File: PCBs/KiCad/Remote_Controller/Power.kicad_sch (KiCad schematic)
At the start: 25 parts

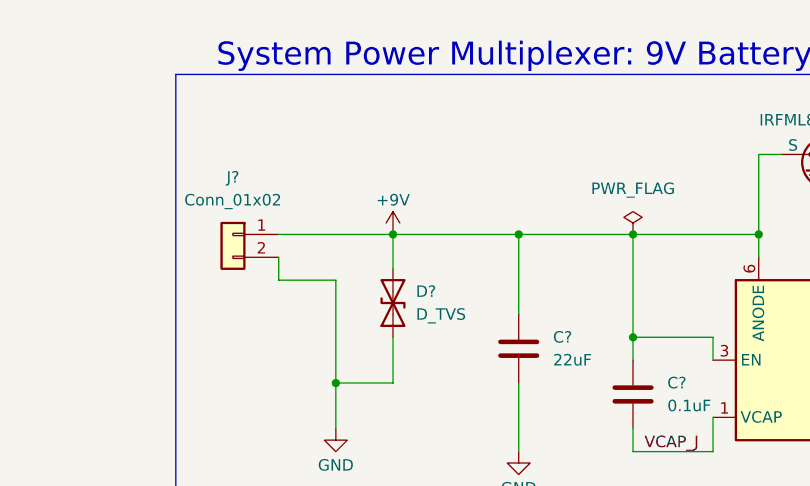
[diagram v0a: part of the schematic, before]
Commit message: Add power switch
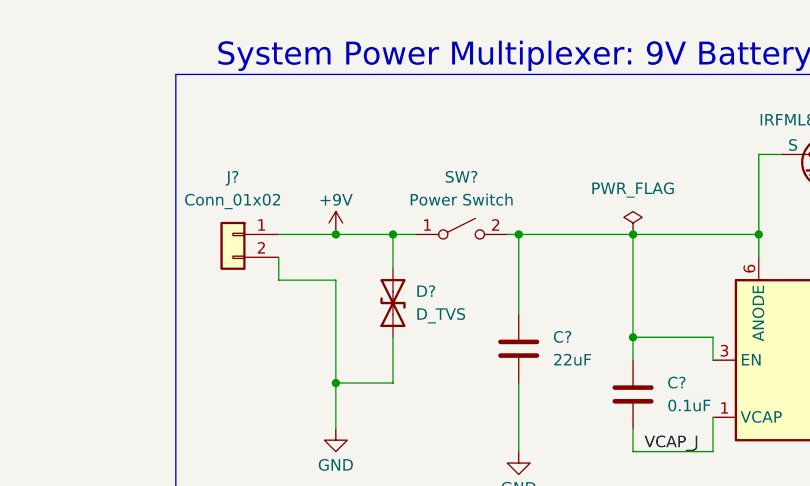
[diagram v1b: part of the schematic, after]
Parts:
- added SW?: Power Switch, symbol Switch:SW_SPST
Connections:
- net +9V: now also SW?.1 (A); no longer C?.1, C?.1, Q?.2 (S), U?.3 (EN), U?.6 (ANODE)
- new net: C?.1, C?.1, Q?.2 (S), SW?.2 (B), U?.3 (EN), U?.6 (ANODE)
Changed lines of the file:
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@@
 	(paper "A4")
 	(junction
-		(at 130.81 170.18)
+		(at 116.84 40.64)
 		(diameter 0)
 		(color 0 0 0 0)
 	)
 	(junction
-		(at 26.67 148.59)
+		(at 130.81 170.18)
 		(diameter 0)
 		(color 0 0 0 0)
 	)
 	(junction
-		(at 143.51 40.64)
+		(at 26.67 148.59)
 		(diameter 0)
 		(color 0 0 0 0)
 	)
 	(junction
-		(at 238.76 55.88)
+		(at 143.51 40.64)
 		(diameter 0)
 		(color 0 0 0 0)
 	)
 	(junction
-		(at 116.84 40.64)
+		(at 238.76 55.88)
 		(diameter 0)
 		(color 0 0 0 0)
@@
 	)
 	(junction
-		(at 102.87 40.64)
-		(diameter 0)
-		(color 0 0 0 0)
-	)
-	(junction
 		(at 106.68 148.59)
 		(diameter 0)
@@
 	)
 	(junction
+		(at 96.52 40.64)
+		(diameter 0)
+		(color 0 0 0 0)
+	)
+	(junction
 		(at 116.84 148.59)
 		(diameter 0)
@@
 	)
 	(junction
+		(at 102.87 40.64)
+		(diameter 0)
+		(color 0 0 0 0)
+	)
+	(junction
 		(at 116.84 95.25)
 		(diameter 0)
@@
 	(wire
 		(pts
-			(xy 102.87 40.64) (xy 116.84 40.64)
-		)
-		(stroke
-			(width 0)
-			(type default)
-		)
-	)
-	(wire
-		(pts
 			(xy 41.91 148.59) (xy 53.34 148.59)
 		)
@@
 	(wire
 		(pts
+			(xy 115.57 40.64) (xy 116.84 40.64)
+		)
+		(stroke
+			(width 0)
+			(type default)
+		)
+	)
+	(wire
+		(pts
 			(xy 231.14 45.72) (xy 220.98 45.72)
 		)
@@
 	(wire
 		(pts
-			(xy 90.17 40.64) (xy 102.87 40.64)
+			(xy 90.17 40.64) (xy 96.52 40.64)
 		)
 		(stroke
@@
 	(wire
 		(pts
+			(xy 102.87 40.64) (xy 105.41 40.64)
+		)
+		(stroke
+			(width 0)
+			(type default)
+		)
+	)
+	(wire
+		(pts
 			(xy 102.87 52.07) (xy 102.87 57.15)
 		)
@@
 	(wire
 		(pts
+			(xy 96.52 40.64) (xy 102.87 40.64)
+		)
+		(stroke
+			(width 0)
+			(type default)
+		)
+	)
+	(wire
+		(pts
 			(xy 220.98 55.88) (xy 238.76 55.88)
 		)
@@
 	(symbol
 		(lib_id "power:+9V")
-		(at 102.87 40.64 0)
+		(at 96.52 40.64 0)
 		(unit 1)
 		(exclude_from_sim no)
@@
 		(dnp no)
 		(property "Reference" "#PWR09"
-			(at 102.87 44.45 0)
+			(at 96.52 44.45 0)
 			(effects
 				(font
@@
 		)
 		(property "Value" "+9V"
-			(at 102.87 36.83 0)
+			(at 96.52 36.83 0)
 			(effects
 				(font
@@
 		)
 		(property "Footprint" ""
-			(at 102.87 40.64 0)
+			(at 96.52 40.64 0)
 			(effects
 				(font
@@
 		)
 		(property "Datasheet" ""
-			(at 102.87 40.64 0)
+			(at 96.52 40.64 0)
 			(effects
 				(font
@@
 		)
 		(property "Description" "Power symbol creates a global label with name \"+9V\""
-			(at 102.87 40.64 0)
+			(at 96.52 40.64 0)
 			(effects
 				(font
@@
 					(unit 1)
 				)
+			)
+		)
+	)
+	(symbol
+		(lib_id "Switch:SW_SPST")
+		(at 110.49 40.64 0)
+		(unit 1)
+		(exclude_from_sim no)
+		(in_bom yes)
+		(on_board yes)
+		(dnp no)
+		(fields_autoplaced yes)
+		(property "Reference" "SW?"
+			(at 110.49 34.29 0)
+			(effects
+				(font
+					(size 1.27 1.27)
+				)
+			)
+		)
+		(property "Value" "Power Switch"
+			(at 110.49 36.83 0)
+			(effects
+				(font
+					(size 1.27 1.27)
+				)
+			)
+		)
+		(property "Footprint" ""
+			(at 110.49 40.64 0)
+			(effects
+				(font
+					(size 1.27 1.27)
+				)
+				(hide yes)
+			)
+		)
+		(property "Datasheet" "~"
+			(at 110.49 40.64 0)
+			(effects
+				(font
+					(size 1.27 1.27)
+				)
+				(hide yes)
+			)
+		)
+		(property "Description" "Single Pole Single Throw (SPST) switch"
+			(at 110.49 40.64 0)
+			(effects
+				(font
+					(size 1.27 1.27)
+				)
+				(hide yes)
+			)
+		)
+		(pin "1"
+		)
+		(pin "2"
+		)
+		(instances
+			(project ""
+				(path "/7afb5074-6b77-4607-a5eb-938c2def45ba/bc757f9b-317d-459c-8896-b31b23ed4983"
+					(reference "SW?")
+					(unit 1)
+				)
